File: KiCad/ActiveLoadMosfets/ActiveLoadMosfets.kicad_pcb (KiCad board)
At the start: 2 copper layers, 30 parts, among them J1 Conn_01x02_Male, Q1 STP60NF06L, Q2 STP60NF06L, Q3 STP60NF06L, Q4 STP60NF06L, Q5 STP60NF06L, Q6 STP60NF06L, U1 LM7322, U2 LM78M12

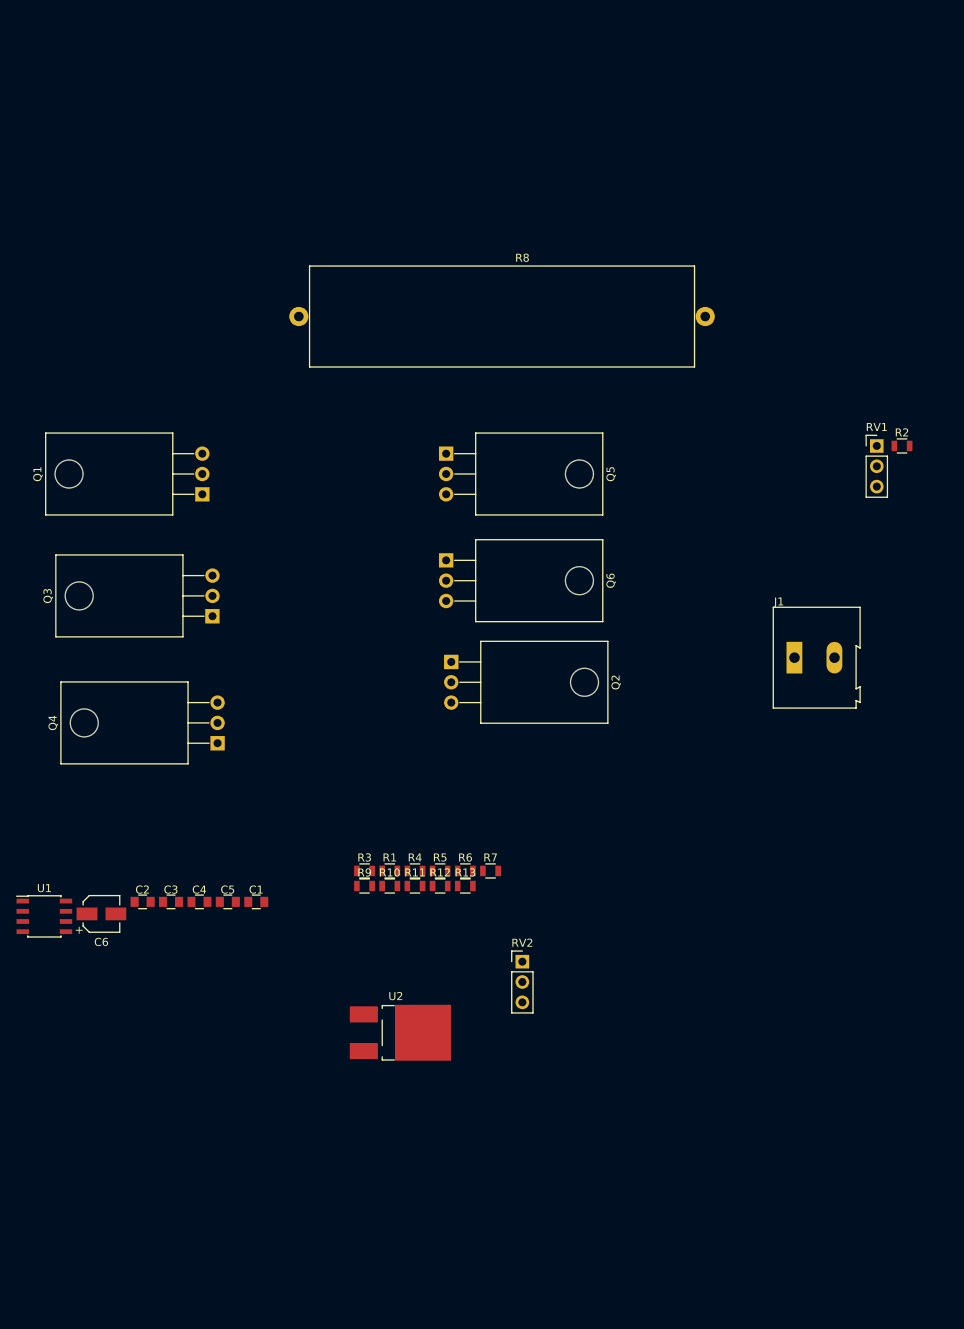
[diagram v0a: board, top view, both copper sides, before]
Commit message: pcb work
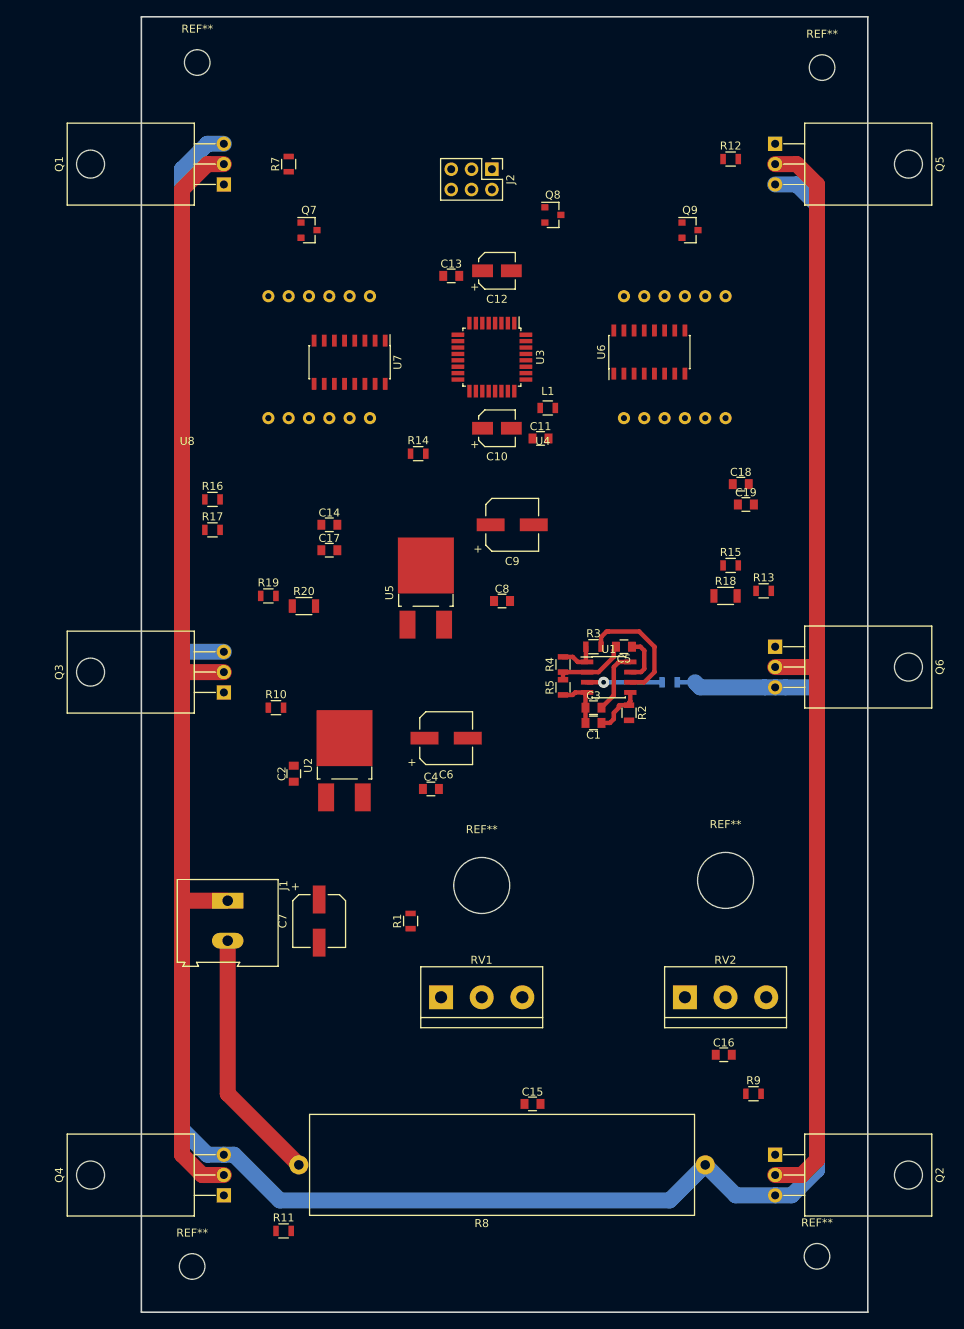
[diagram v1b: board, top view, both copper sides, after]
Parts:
- added C10: 10u, Capacitors_SMD:CP_Elec_4x5.8, F.Cu at (106.0, 64.8)
- added C11: 100n, Capacitors_SMD:C_0805, F.Cu at (111.5, 66.0)
- added C12: 10u, Capacitors_SMD:CP_Elec_4x5.8, F.Cu at (106.0, 45.1)
- added C13: 100n, Capacitors_SMD:C_0805, F.Cu at (100.3, 45.7)
- added C14: 10n, Capacitors_SMD:C_0805, F.Cu at (85.1, 76.8)
- added C15: 100n, Capacitors_SMD:C_0805, F.Cu at (110.5, 149.2)
- added C16: 100n, Capacitors_SMD:C_0805, F.Cu at (134.4, 143.1)
- added C17: 1u, Capacitors_SMD:C_0805, F.Cu at (85.1, 80.0)
- added C18: 1u, Capacitors_SMD:C_0805, F.Cu at (136.5, 71.8)
- added C19: 10n, Capacitors_SMD:C_0805, F.Cu at (137.2, 74.3)
- added C7: 47u, Capacitors_SMD:CP_Elec_6.3x5.8, F.Cu at (83.8, 126.4)
- added C8: 100n, Capacitors_SMD:C_0805, F.Cu at (106.7, 86.4)
- added C9: 47u, Capacitors_SMD:CP_Elec_6.3x5.8, F.Cu at (108.0, 76.8)
- added J2: Conn_02x03_Odd_Even, Pin_Headers:Pin_Header_Straight_2x03_Pitch2.54mm, F.Cu at (105.4, 32.4)
- added L1: 10u, Inductors_SMD:L_0805, F.Cu at (112.4, 62.2)
- added Q7: IRLML2244, TO_SOT_Packages_SMD:SOT-23, F.Cu at (82.5, 40.0)
- added Q8: IRLML2244, TO_SOT_Packages_SMD:SOT-23, F.Cu at (113.0, 38.1)
- added Q9: IRLML2244, TO_SOT_Packages_SMD:SOT-23, F.Cu at (130.2, 40.0)
- added R14: 10k, Resistors_SMD:R_0805, F.Cu at (96.2, 67.9)
- added R15: 1k, Resistors_SMD:R_0805, F.Cu at (135.3, 81.9)
- added R16: 1k, Resistors_SMD:R_0805, F.Cu at (70.5, 73.7)
- added R17: 1k, Resistors_SMD:R_0805, F.Cu at (70.5, 77.5)
- added R18: 10, Resistors_SMD:R_1206, F.Cu at (134.6, 85.7)
- added R19: 1k, Resistors_SMD:R_0805, F.Cu at (77.5, 85.7)
- added R20: 10, Resistors_SMD:R_1206, F.Cu at (81.9, 87.0)
- added REF**: MountingHole_6mm, Mounting_Holes:MountingHole_6mm, F.Cu at (104.1, 121.9)
- added REF**: MountingHole_6mm, Mounting_Holes:MountingHole_6mm, F.Cu at (134.6, 121.3)
- added REF**: MountingHole_3.2mm_M3, Mounting_Holes:MountingHole_3.2mm_M3, F.Cu at (67.9, 169.5)
- added REF**: MountingHole_3.2mm_M3, Mounting_Holes:MountingHole_3.2mm_M3, F.Cu at (146.1, 168.3)
- added REF**: MountingHole_3.2mm_M3, Mounting_Holes:MountingHole_3.2mm_M3, F.Cu at (146.7, 19.7)
- added REF**: MountingHole_3.2mm_M3, Mounting_Holes:MountingHole_3.2mm_M3, F.Cu at (68.6, 19.1)
- added U3: ATxmega32E5-AU, Housings_QFP:TQFP-32_7x7mm_Pitch0.8mm, F.Cu at (105.4, 55.9)
- added U4: LED-3digits, JPDisplays:LED-14.2x3, F.Cu at (128.3, 55.9)
- added U5: LM78M33, TO_SOT_Packages_SMD:TO-252-2_Rectifier, F.Cu at (97.2, 84.7)
- added U6: SCT2167, Housings_SOIC:SOIC-16_3.9x9.9mm_Pitch1.27mm, F.Cu at (125.1, 55.2)
- added U7: SCT2167, Housings_SOIC:SOIC-16_3.9x9.9mm_Pitch1.27mm, F.Cu at (87.6, 56.5)
- added U8: LED-3digits, JPDisplays:LED-14.2x3, F.Cu at (83.8, 55.9)
- C6: value 10u -> 47u; footprint Capacitors_SMD:CP_Elec_4x5.8 -> Capacitors_SMD:CP_Elec_6.3x5.8
- R6: moved to B.Cu
- RV1, RV2: footprint Pin_Headers:Pin_Header_Straight_1x03_Pitch2.54mm -> Connectors_Terminal_Blocks:TerminalBlock_bornier-3_P5.08mm
- moved R8 117.6 mm to (132.1, 156.8), turned to 180 degrees
- moved R12 97.9 mm to (135.3, 31.1)
- moved R7 91.9 mm to (80.0, 31.8), turned to 90 degrees
- moved RV1 87.8 mm to (99.1, 135.9)
- moved J1 77.1 mm to (72.4, 123.8), turned to 270 degrees
- moved U1 76.6 mm to (120.0, 95.9)
- moved Q2 73.7 mm to (140.8, 155.6)
- moved C5 58.9 mm to (121.9, 92.1), turned to 180 degrees
- moved C3 58.1 mm to (118.1, 99.7)
- moved Q4 56.5 mm to (71.9, 160.7)
- moved Q5 56.5 mm to (140.8, 29.2)
- moved R9 55.1 mm to (138.1, 148.0)
- moved R13 52.5 mm to (139.4, 85.1)
- moved C6 48.4 mm to (99.7, 103.5)
- moved C1 47.7 mm to (118.1, 101.6), turned to 180 degrees
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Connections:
- net Net-(Q1-Pad3) renamed CURRENT
- RV2 pad 1: (no net) -> Net-(RV2-Pad1)
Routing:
- net CURRENT: track 0.00 -> 364.2 mm
- net VDD: track 0.00 -> 283.9 mm
- net GND: track 0.00 -> 39.2 mm
- net Net-(R3-Pad2): track 0.00 -> 15.7 mm
- net Net-(C5-Pad2): track 0.00 -> 9.48 mm
- net Net-(R6-Pad2): track 0.00 -> 9.37 mm, vias 0 -> 1
- net +12V: track 0.00 -> 8.05 mm
- net Net-(C1-Pad1): track 0.00 -> 6.63 mm
- net Net-(C5-Pad1): track 0.00 -> 5.94 mm
- net Net-(R3-Pad1): track 0.00 -> 5.25 mm
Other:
- board outline added: 90.8 x 161.9 mm
- net class Default: trace_width 0.25 -> 0.5588; via_dia 0.8 -> 1.4; via_drill 0.4 -> 0.6
- net class Power added: clearance 0.2, trace_width 2, via_dia 2, via_drill 0.8
